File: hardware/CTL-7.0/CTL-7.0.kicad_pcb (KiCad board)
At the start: 2 copper layers, 18 parts, among them J2 Left, J3 Right, U1 STM32H750VBTx, U2 AMS1117-3.3, Y1 32.768K, Y2 25MHz

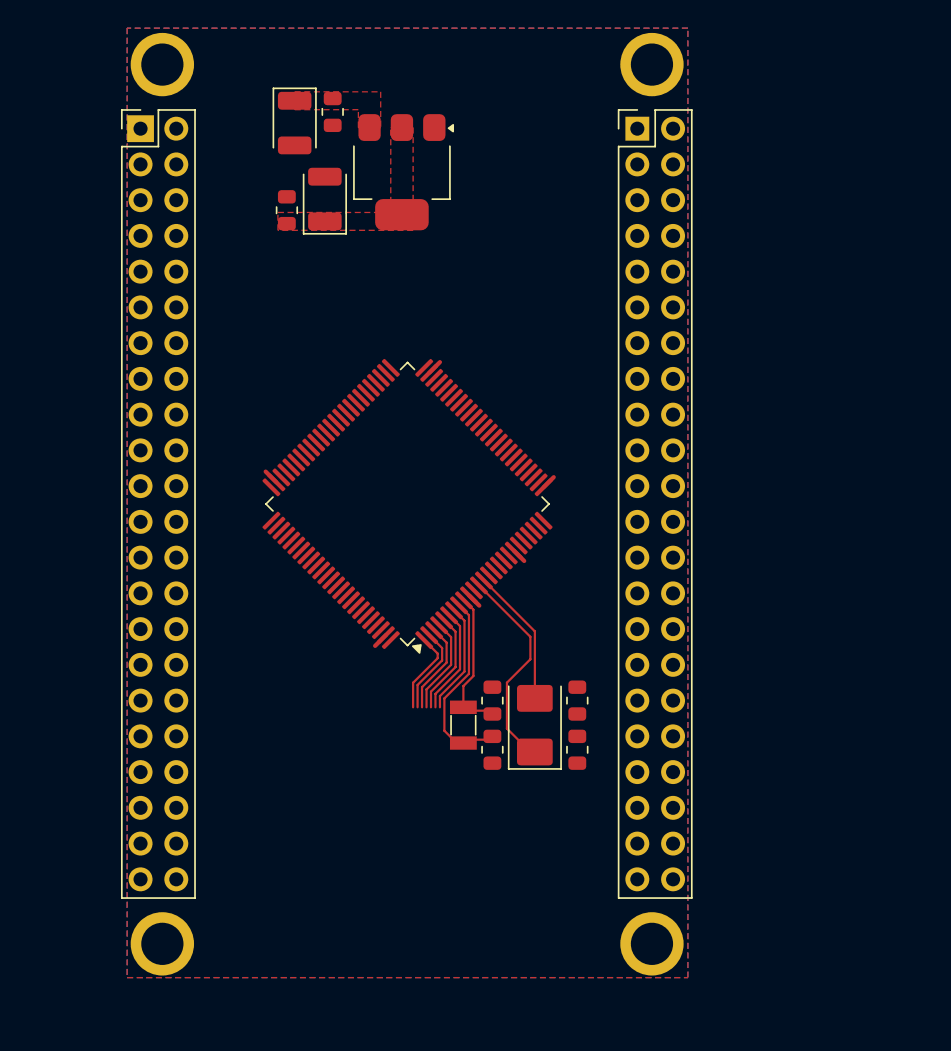
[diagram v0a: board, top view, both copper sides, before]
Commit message: modified:   Ferrite Transformer Calculation.xlsx 	modified:   archive/Peripheral Migration ESP32S3-STM32H7.md 	renamed:    archive/PR_ 0201_2026.docx -> archive/Purchase 20260201.docx 	new file:   archive/Purchase 20260720.docx 	new file:   archive/Purchase Plan/bom.csv 	new file:   archive/Purchase Plan/bom.xlsx 	new file:   archive/Purchase Recaps.xlsx 	modified:   archive/REM - Vsense.xlsx 	new file:   archive/datasheets/SPC7040.PDF 	new file:   archive/datasheets/rm0433-stm32h742-stm32h743-753-and-stm32h750-value-line-advanced-armbased-32bit-mcus-stmicroelectronics.pdf 	new file:   archive/refferences/MiniSTM32H7xx-master/.gitattributes 	new file:   archive/refferences/MiniSTM32H7xx-master/.gitignore 	new file:   archive/refferences/MiniSTM32H7xx-master/Datasheet/MCU/DM00287603_ZHV2.pdf 	new file:   "archive/refferences/MiniSTM32H7xx-master/Datasheet/MCU/ES0396_STM32H750xB\345\222\214STM32H753xI\345\215\225\347\211\207\346\234\272\347\232\204\345\261\200\351\231\220\346\200\247.pdf" 	new file:   "archive/refferences/MiniSTM32H7xx-master/Datasheet/MCU/PM0253_STM32F7\345\222\214 STM32H7\345\215\225\347\211\207\346\234\272\347\274\226\347\250\213\346\211\213\345\206\214.pdf" 	new file:   "archive/refferences/MiniSTM32H7xx-master/Datasheet/MCU/RM0433_STM32H7x3\345\222\214STM32H750\345\215\225\347\211\207\346\234\272\345\217\202\350\200\203\346\211\213\345\206\214.pdf" 	new file:   archive/refferences/MiniSTM32H7xx-master/Datasheet/MCU/STM32H743VI_Datasheet.pdf 	new file:   archive/refferences/MiniSTM32H7xx-master/Datasheet/MCU/STM32H750VB_Datasheet.pdf 	new file:   archive/refferences/MiniSTM32H7xx-master/Datasheet/MKESD0402MS05.PDF 	new file:   archive/refferences/MiniSTM32H7xx-master/Datasheet/ST7735S_V1.5_20150303.pdf 	new file:   archive/refferences/MiniSTM32H7xx-master/Datasheet/SY8088AAC.PDF 	new file:   archive/refferences/MiniSTM32H7xx-master/Datasheet/Sensor/OV2640-camera module.pdf 	new file:   archive/refferences/MiniSTM32H7xx-master/Datasheet/Sensor/OV26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
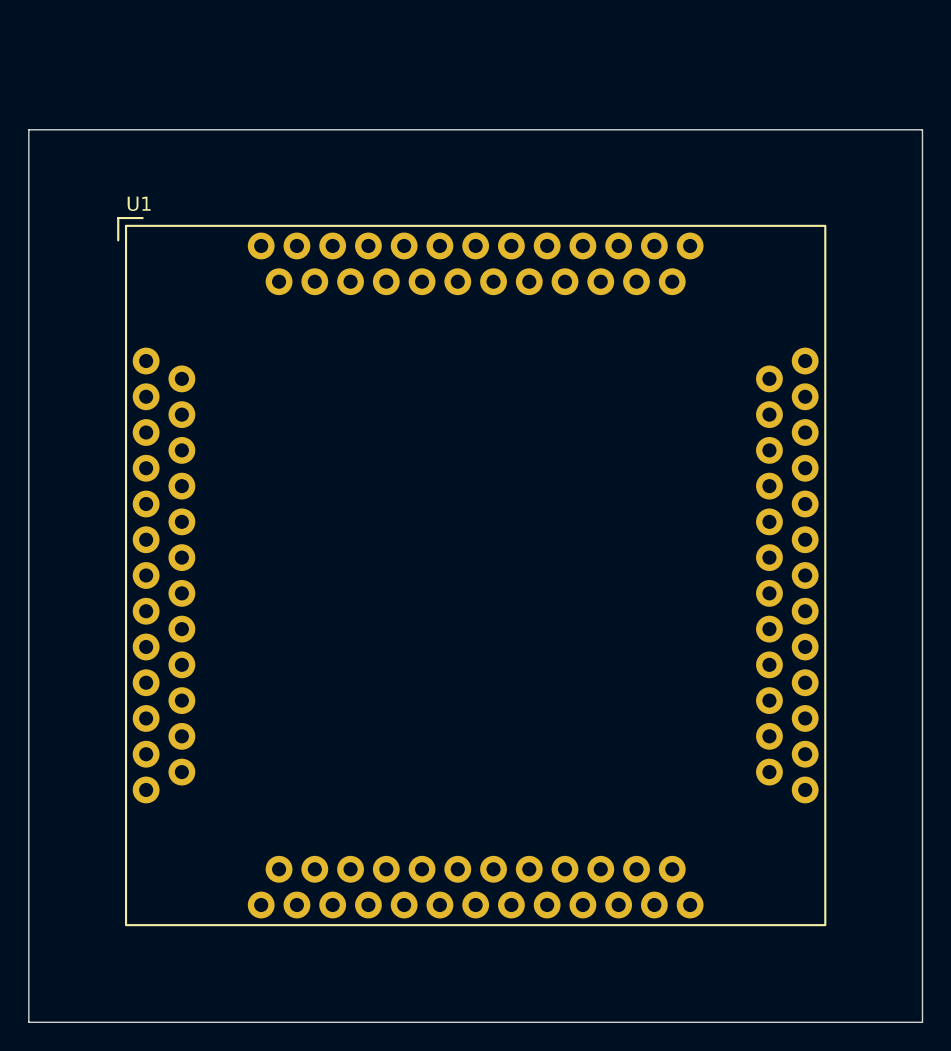
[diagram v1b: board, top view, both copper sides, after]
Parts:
- removed C1, C3: 10u, Capacitor_Tantalum_SMD:CP_EIA-3528-12_Kemet-T
- removed C2, C4: 100n, Capacitor_SMD:C_0805_2012Metric
- removed C5, C6: 10p, Capacitor_SMD:C_0805_2012Metric
- removed C7, C8: 20p, Capacitor_SMD:C_0805_2012Metric
- removed H1, H2, H3, H4: MountingHole_Pad, MountingHole:MountingHole_3mm_Pad
- removed J2: Left, Connector_PinHeader_2.54mm:PinHeader_2x22_P2.54mm_Vertical
- removed J3: Right, Connector_PinHeader_2.54mm:PinHeader_2x22_P2.54mm_Vertical
- removed U2: AMS1117-3.3, Package_TO_SOT_SMD:SOT-223-3_TabPin2
- removed Y1: 32.768K, Crystal:Crystal_SMD_3215-2Pin_3.2x1.5mm
- removed Y2: 25MHz, Crystal:Crystal_SMD_5032-2Pin_5.0x3.2mm
- U1: value STM32H750VBTx -> H750; footprint Package_QFP:LQFP-100_14x14mm_P0.5mm -> Core:STM32H750_v1
- moved U1 7.02 mm to (131.8, 98.2), turned to 0 degrees
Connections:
- U1 pad 100: +3.3V -> Net-(U1-+3.3V-Pad100)
- U1 pad 11: +3.3V -> Net-(U1-+3.3V-Pad100)
- U1 pad 12: Net-(U1-PH0) -> (no net)
- U1 pad 13: Net-(U1-PH1) -> (no net)
- U1 pad 21: unconnected-(U1-VDDA-Pad21) -> (no net)
- U1 pad 27: +3.3V -> Net-(U1-+3.3V-Pad100)
- U1 pad 50: +3.3V -> unconnected-(U1-+5V-Pad50)
- U1 pad 75: +3.3V -> Net-(U1-+3.3V-Pad100)
- U1 pad 8: Net-(U1-PC14) -> (no net)
- U1 pad 9: Net-(U1-PC15) -> (no net)
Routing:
- net Net-(U1-PH0): track 13.6 -> 0.00 mm
- net Net-(U1-PC14): track 12.4 -> 0.00 mm
- net Net-(U1-PC15): track 10.3 -> 0.00 mm
- net Net-(U1-PH1): track 9.88 -> 0.00 mm
- net unconnected-(U1-PC13-Pad7): track 7.93 -> 0.00 mm
- net unconnected-(U1-VBAT-Pad6): track 7.59 -> 0.00 mm
- net unconnected-(U1-PE6-Pad5): track 7.25 -> 0.00 mm
- net unconnected-(U1-PE5-Pad4): track 6.91 -> 0.00 mm
- net unconnected-(U1-PE4-Pad3): track 6.57 -> 0.00 mm
- net GND: track 6.35 -> 0.00 mm
- net unconnected-(U1-PE3-Pad2): track 6.24 -> 0.00 mm
- net unconnected-(U1-PE2-Pad1): track 5.90 -> 0.00 mm
- removed copper zone on F.Cu, net +3.3V
- removed copper zone on F.Cu, net +5V
- removed copper zone on B.Cu, net GND
- removed copper zone on F.Cu, net GND
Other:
- board outline added: 63.5 x 63.4 mm
